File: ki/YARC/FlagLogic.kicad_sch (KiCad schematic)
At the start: 13 parts, among them U105 74LS86, U106 74LS139, U107 74HC00, U108 74HC02, U109 74LS32, U110 74LS21, U111 74LS153, U112 74LS573, U113 74LS573, U114 74LS574, U115 74LS574, U135 74HC02, U136 74LS32

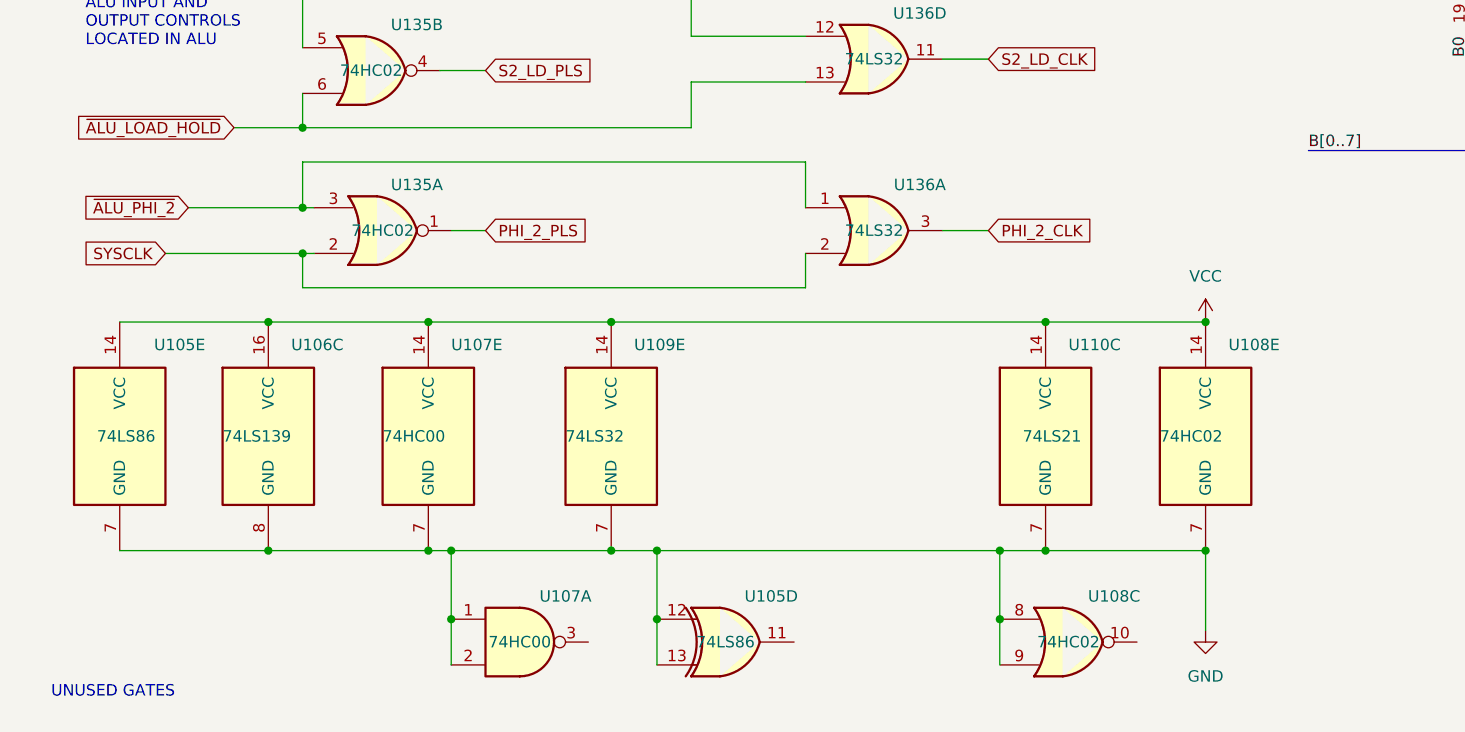
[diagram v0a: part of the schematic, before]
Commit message: Ongoing corrections and improvements
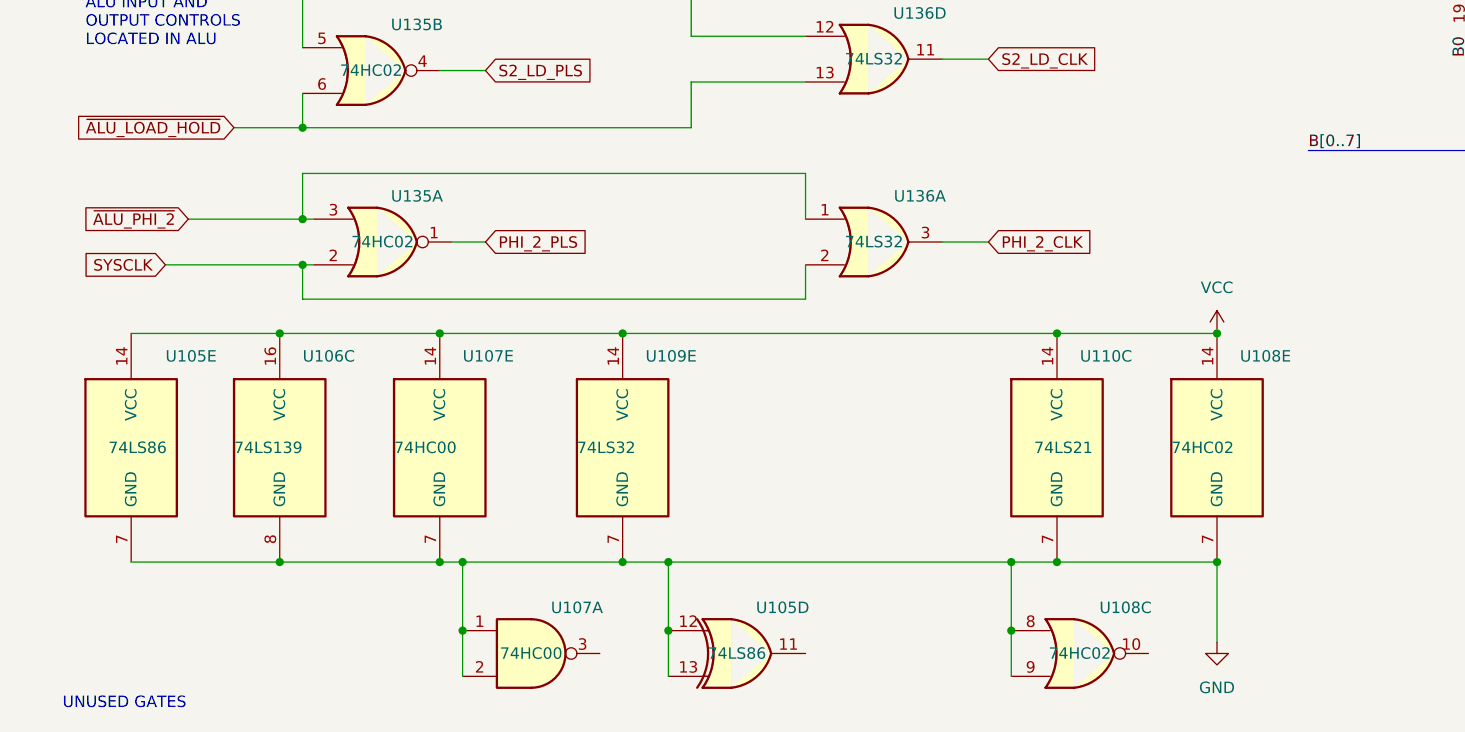
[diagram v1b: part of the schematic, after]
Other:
- moved on the sheet: U105D, U105E, U106C, U107A, U107E, U108C, U108E, U109E, U110C, U135A, U136A
